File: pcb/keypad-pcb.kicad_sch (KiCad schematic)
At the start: 16 parts, among them SW1 SW_Push, U1 ATmega32U4-A, Y1 Crystal_GND24_Small

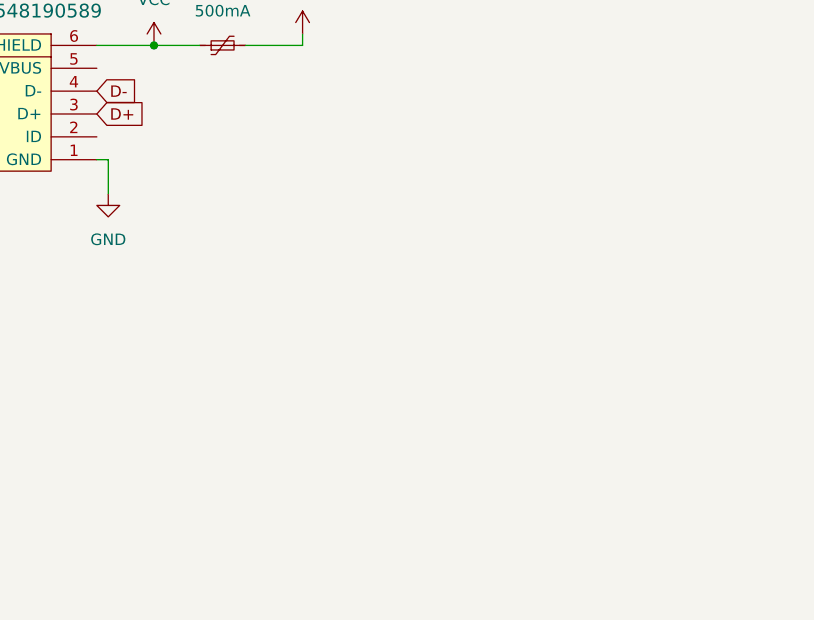
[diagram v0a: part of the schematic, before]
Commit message: schematic complete
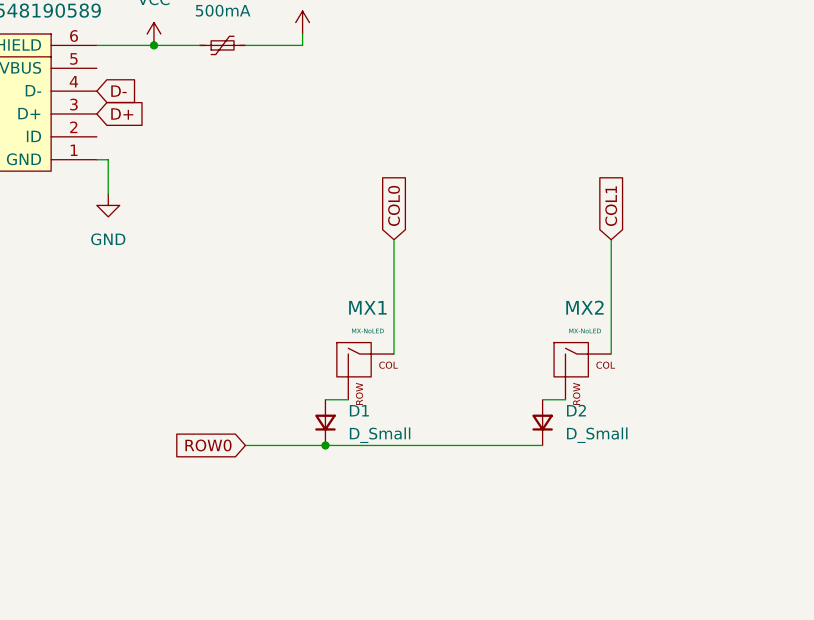
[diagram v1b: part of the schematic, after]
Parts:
- added D1, D2: D_Small, symbol Device:D_Small
- added MX1, MX2: MX-NoLED, symbol MX_Alps_Hybrid:MX-NoLED
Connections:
- new net: D1.2 (A), MX1.2 (ROW)
- new net: D2.2 (A), MX2.2 (ROW)
- new net COL0: MX1.1 (COL)
- new net COL1: MX2.1 (COL)
- new net ROW0: D1.1 (K), D2.1 (K)
